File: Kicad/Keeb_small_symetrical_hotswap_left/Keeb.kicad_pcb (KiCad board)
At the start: 2 copper layers, 96.3 x 99.3 mm, 20 parts, among them J1 TYPE-C-31-M-12, SW1 CherryMX, SW10 CherryMX, SW11 CherryMX, SW13 CherryMX, SW14 CherryMX, SW15 CherryMX, SW16 CherryMX, SW17 CherryMX, SW18 CherryMX, SW19 CherryMX, SW20 CherryMX, SW3 CherryMX, SW4 CherryMX, SW5 CherryMX, SW6 CherryMX, SW7 CherryMX, SW8 CherryMX, SW9 CherryMX, U1 Pico

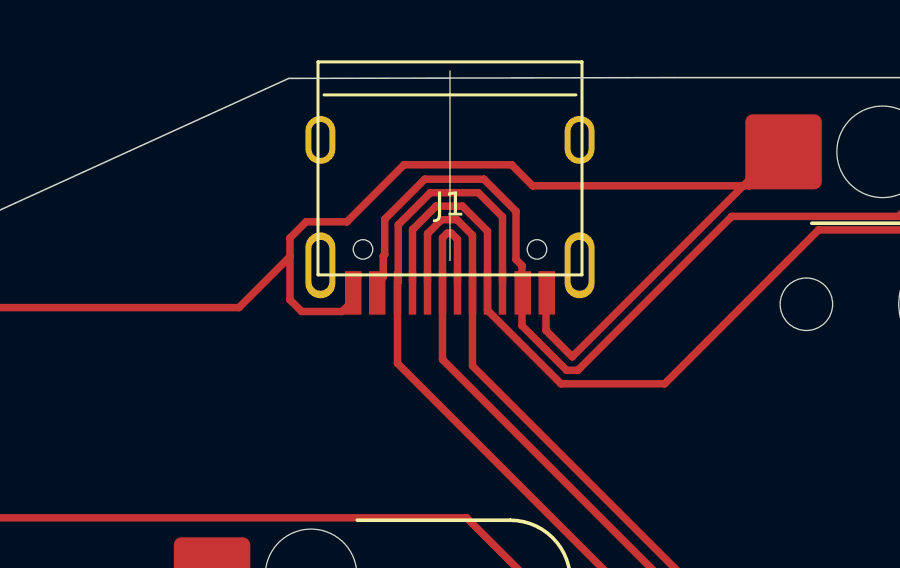
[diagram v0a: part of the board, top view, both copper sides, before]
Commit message: min
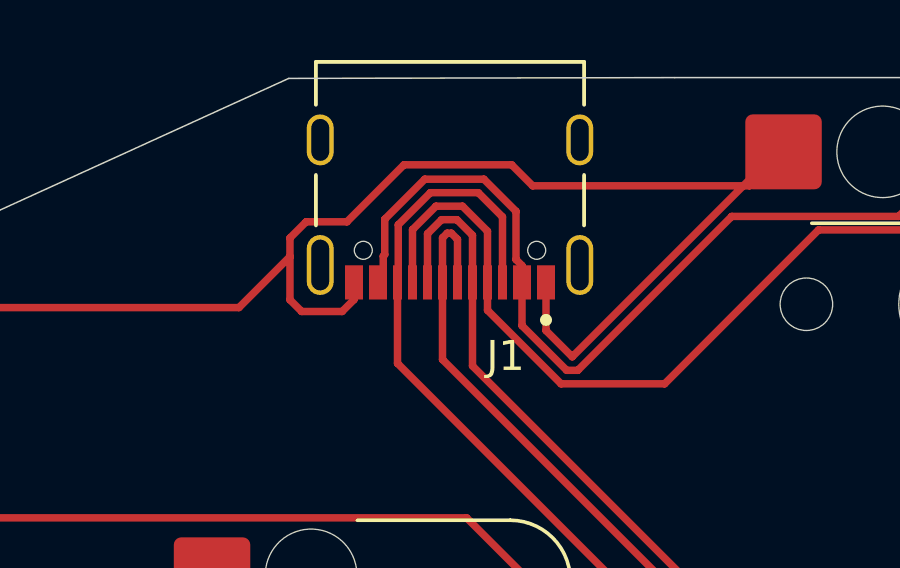
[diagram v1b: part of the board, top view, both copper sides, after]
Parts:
- J1: footprint USB-C-Power-tester:TYPE-C-31-M-12 -> TypeC:HRO_TYPE-C-31-M-12
